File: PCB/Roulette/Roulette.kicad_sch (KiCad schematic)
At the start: 185 parts, among them J2 Shelly, J2 USB-PROG, SW1 SW_Push, U2 ESP32-S3-MINI-1

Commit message: Parts - needs text and artwork
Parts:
- SW1: LCSC Part # (none) -> C520860
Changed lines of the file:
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@@
+      (effects (font (size 1.27 1.27)) hide)
+    )
+    (property "LCSC Part #" "C520860" (at 247.65 64.135 0)
       (effects (font (size 1.27 1.27)) hide)
     )
@@
       (effects (font (size 1.27 1.27)) hide)
     )
+    (property "LCSC Part #" "C520860" (at 247.65 90.17 0)
+      (effects (font (size 1.27 1.27)) hide)
+    )

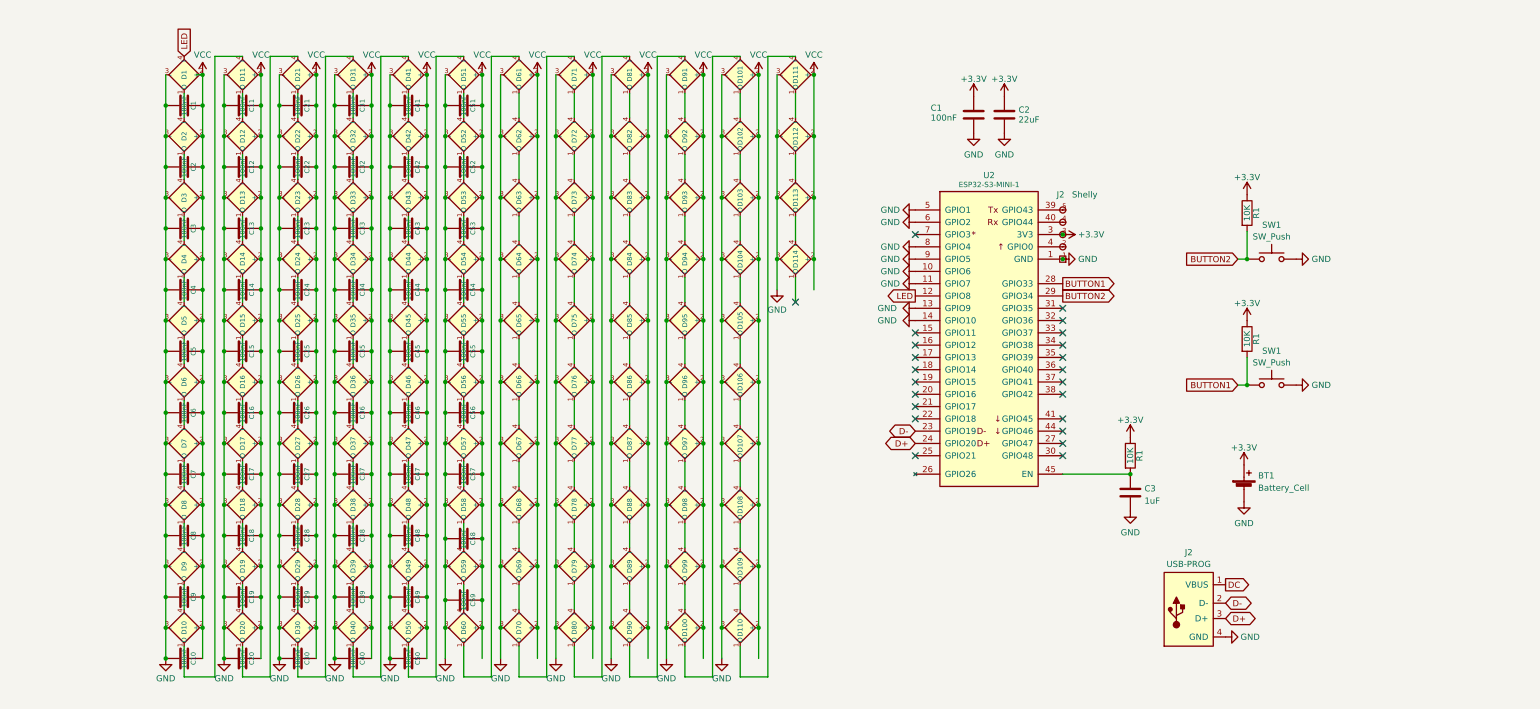
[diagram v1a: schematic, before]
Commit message: First attempt
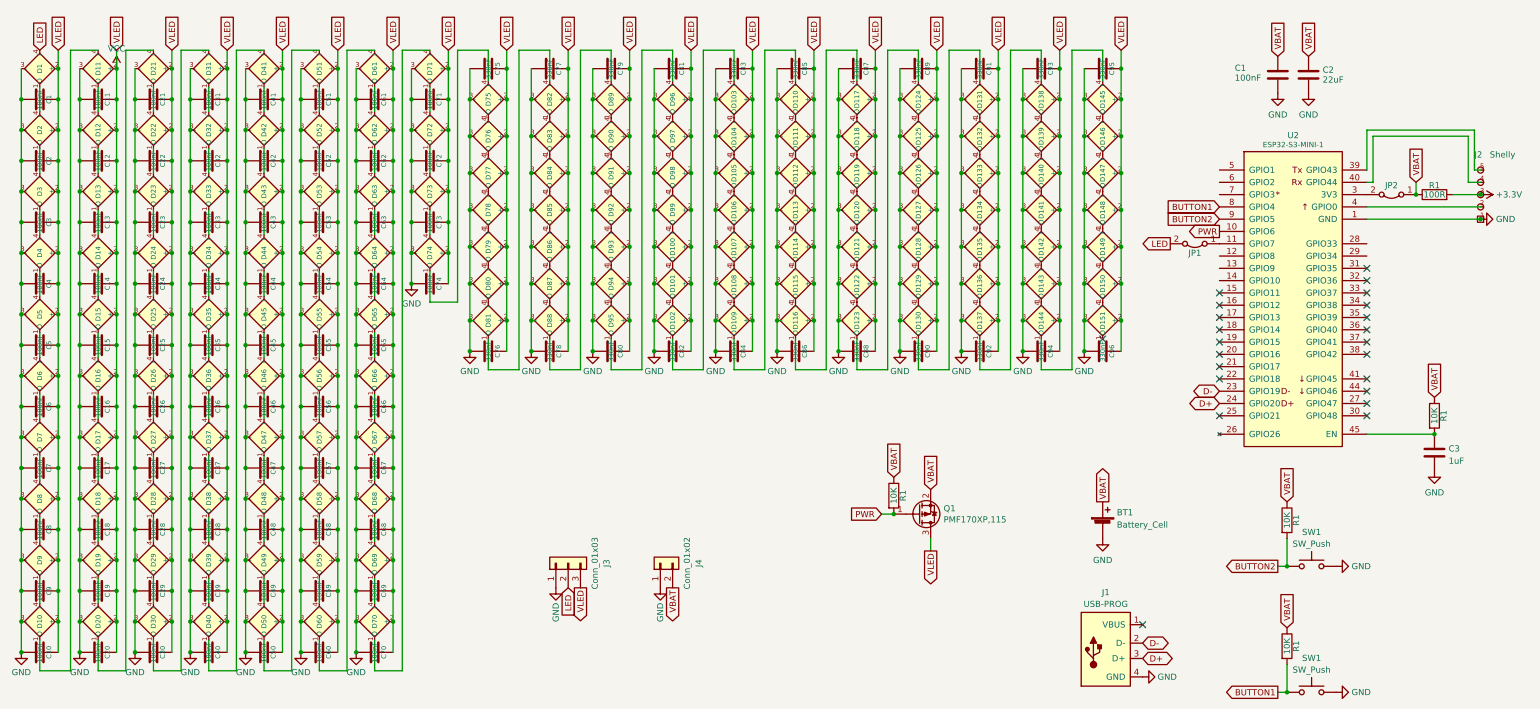
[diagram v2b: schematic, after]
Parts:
- added C60, C61, C62, C63, C64, C65, C66, C67, C68, C69, C70, C71, C72, C73, C74: 100nF, RevK:C_0402, symbol Device:C
- added C75, C76, C77, C78, C79, C80, C81, C82, C83, C84, C85, C86, C87, C88, C89, C90, C91, C92, C93, C94, C95, C96: 330nF, RevK:C_0402, symbol Device:C
- added D115, D116, D117, D118, D119, D120, D121, D122, D123, D124, D125, D126, D127, D128, D129, D130, D131, D132, D133, D134, D135, D136, D137, D138, D139, D140, D141, D142, D143, D144, D145, D146, D147, D148, D149, D150, D151: XL-1010RGBC-WS2812B, RevK:SMD1010, symbol RevK:WS2812B-1mm
- added J3: Conn_01x03, RevK:3-PADS, symbol Connector_Generic:Conn_01x03
- added J4: Conn_01x02, RevK:2-PADS, symbol Connector_Generic:Conn_01x02
- added JP1, JP2: Jumper_2_Bridged, RevK:Pad_1206_0805_Bridged, symbol Jumper:Jumper_2_Bridged
- added Q1: PMF170XP,115, RevK:SOT-323_SC-70, symbol Device:Q_PMOS_GSD
- added R1: 100R, RevK:R_0402, symbol Device:R
- added R1: 10K, RevK:R_0402, symbol Device:R
- renumbered J2 to J1
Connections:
- net +3V3: now also R1.2; no longer BT1.1 (+), C1.1, C2.1, R1.1, R1.1, R1.1, U2.3 (3V3)
- net BUTTON1: now also U2.8 (GPIO4); no longer U2.28 (GPIO33)
- net BUTTON2: now also U2.9 (GPIO5); no longer U2.29 (GPIO34)
- net GND: now also C60.2, C61.2, C62.2, C63.2, C64.2, C65.2, C66.2, C67.2, C68.2, C69.2, C70.2, C71.2, C72.2, C73.2, C74.2, C75.2, C76.2, C77.2, C78.2, C79.2, C80.2, C81.2, C82.2, C83.2, C84.2, C85.2, C86.2, C87.2, C88.2, C89.2, C90.2, C91.2, C92.2, C93.2, C94.2, C95.2, C96.2, D115.3 (-), D116.3 (-), D117.3 (-), D118.3 (-), D119.3 (-), D120.3 (-), D121.3 (-), D122.3 (-), D123.3 (-), D124.3 (-), D125.3 (-), D126.3 (-), D127.3 (-), D128.3 (-), D129.3 (-), D130.3 (-), D131.3 (-), D132.3 (-), D133.3 (-), D134.3 (-), D135.3 (-), D136.3 (-), D137.3 (-), D138.3 (-), D139.3 (-), D140.3 (-), D141.3 (-), D142.3 (-), D143.3 (-), D144.3 (-), D145.3 (-), D146.3 (-), D147.3 (-), D148.3 (-), D149.3 (-), D150.3 (-), D151.3 (-), J3.1 (Pin_1), J4.1 (Pin_1); no longer U2.10 (GPIO6), U2.11 (GPIO7), U2.13 (GPIO9), U2.14 (GPIO10), U2.5 (GPIO1), U2.6 (GPIO2), U2.8 (GPIO4), U2.9 (GPIO5)
- net LED: now also J3.2 (Pin_2), JP1.2 (B); no longer U2.12 (GPIO8)
- net VCC: now also C60.1, C61.1, C62.1, C63.1, C64.1, C65.1, C66.1, C67.1, C68.1, C69.1, C70.1, C71.1, C72.1, C73.1, C74.1, C75.1, C76.1, C77.1, C78.1, C79.1, C80.1, C81.1, C82.1, C83.1, C84.1, C85.1, C86.1, C87.1, C88.1, C89.1, C90.1, C91.1, C92.1, C93.1, C94.1, C95.1, C96.1, D115.2 (+), D116.2 (+), D117.2 (+), D118.2 (+), D119.2 (+), D120.2 (+), D121.2 (+), D122.2 (+), D123.2 (+), D124.2 (+), D125.2 (+), D126.2 (+), D127.2 (+), D128.2 (+), D129.2 (+), D130.2 (+), D131.2 (+), D132.2 (+), D133.2 (+), D134.2 (+), D135.2 (+), D136.2 (+), D137.2 (+), D138.2 (+), D139.2 (+), D140.2 (+), D141.2 (+), D142.2 (+), D143.2 (+), D144.2 (+), D145.2 (+), D146.2 (+), D147.2 (+), D148.2 (+), D149.2 (+), D150.2 (+), D151.2 (+), J3.3 (Pin_3), Q1.3 (D)
- net at D114.1 (O): now also D115.4 (I)
- net DC: no longer names the net of J1.1 (VBUS)
- new net: D140.1 (O), D141.4 (I)
- new net: D139.1 (O), D140.4 (I)
- new net: D128.1 (O), D129.4 (I)
- new net: D127.1 (O), D128.4 (I)
- new net: D123.1 (O), D124.4 (I)
- new net: D122.1 (O), D123.4 (I)
- new net: D136.1 (O), D137.4 (I)
- new net: D135.1 (O), D136.4 (I)
- new net: D133.1 (O), D134.4 (I)
- new net: D132.1 (O), D133.4 (I)
- new net: D150.1 (O), D151.4 (I)
- new net: JP2.2 (B), U2.3 (3V3)
- new net: D147.1 (O), D148.4 (I)
- new net: D146.1 (O), D147.4 (I)
- new net: D129.1 (O), D130.4 (I)
- new net: D125.1 (O), D126.4 (I)
- new net: D124.1 (O), D125.4 (I)
- new net: D119.1 (O), D120.4 (I)
- new net: D118.1 (O), D119.4 (I)
- new net: D134.1 (O), D135.4 (I)
- new net: JP1.1 (A), U2.11 (GPIO7)
- new net: D137.1 (O), D138.4 (I)
- new net: D131.1 (O), D132.4 (I)
- new net: D126.1 (O), D127.4 (I)
- new net: D121.1 (O), D122.4 (I)
- new net: D115.1 (O), D116.4 (I)
- new net: D141.1 (O), D142.4 (I)
- new net: D145.1 (O), D146.4 (I)
- new net: D144.1 (O), D145.4 (I)
- new net: D142.1 (O), D143.4 (I)
- new net: D130.1 (O), D131.4 (I)
- new net: D148.1 (O), D149.4 (I)
- new net: D143.1 (O), D144.4 (I)
- new net: D120.1 (O), D121.4 (I)
- new net: D149.1 (O), D150.4 (I)
- new net: D116.1 (O), D117.4 (I)
- new net: D117.1 (O), D118.4 (I)
- new net: D138.1 (O), D139.4 (I)
- new net PWR: Q1.1 (G), R1.2, U2.10 (GPIO6)
- new net VBAT: BT1.1 (+), C1.1, C2.1, J4.2 (Pin_2), JP2.1 (A), Q1.2 (S), R1.1, R1.1, R1.1, R1.1, R1.1
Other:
- moved on the sheet: BT1, C1, C2, C3, J1, J2, R1, SW1, U2
